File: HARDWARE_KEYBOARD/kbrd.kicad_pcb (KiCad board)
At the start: 2 copper layers, 70 x 50 mm, 24 parts, among them J1 USB_C_Receptacle_USB2.0_16P, J2 SWD, SW1 SW_SPST, SW2 SW_SPST, SW3 SW_SPST, SW4 SW_SPST, U1 STM32F103C8Tx, U2 AP2210N-3.3TRG1, Y1 Crystal_GND24

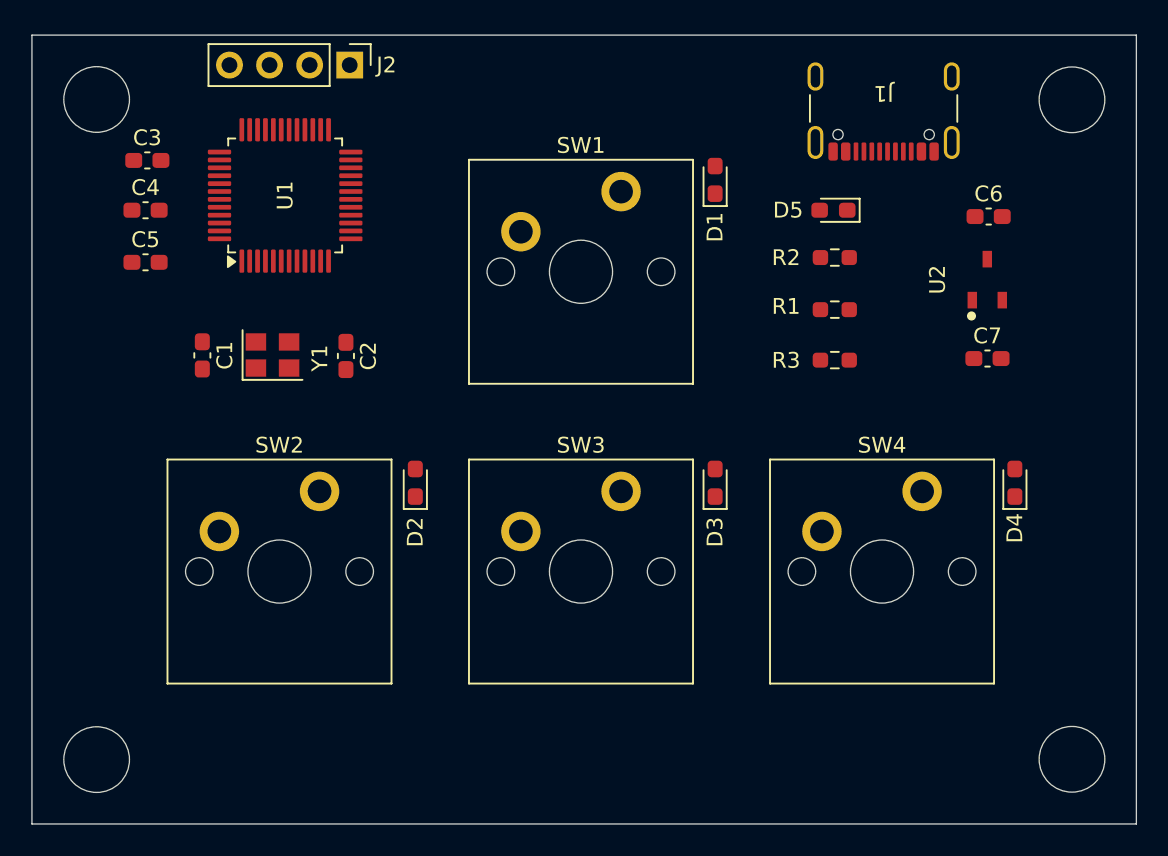
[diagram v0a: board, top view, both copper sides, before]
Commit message: Updated PCB & schematic
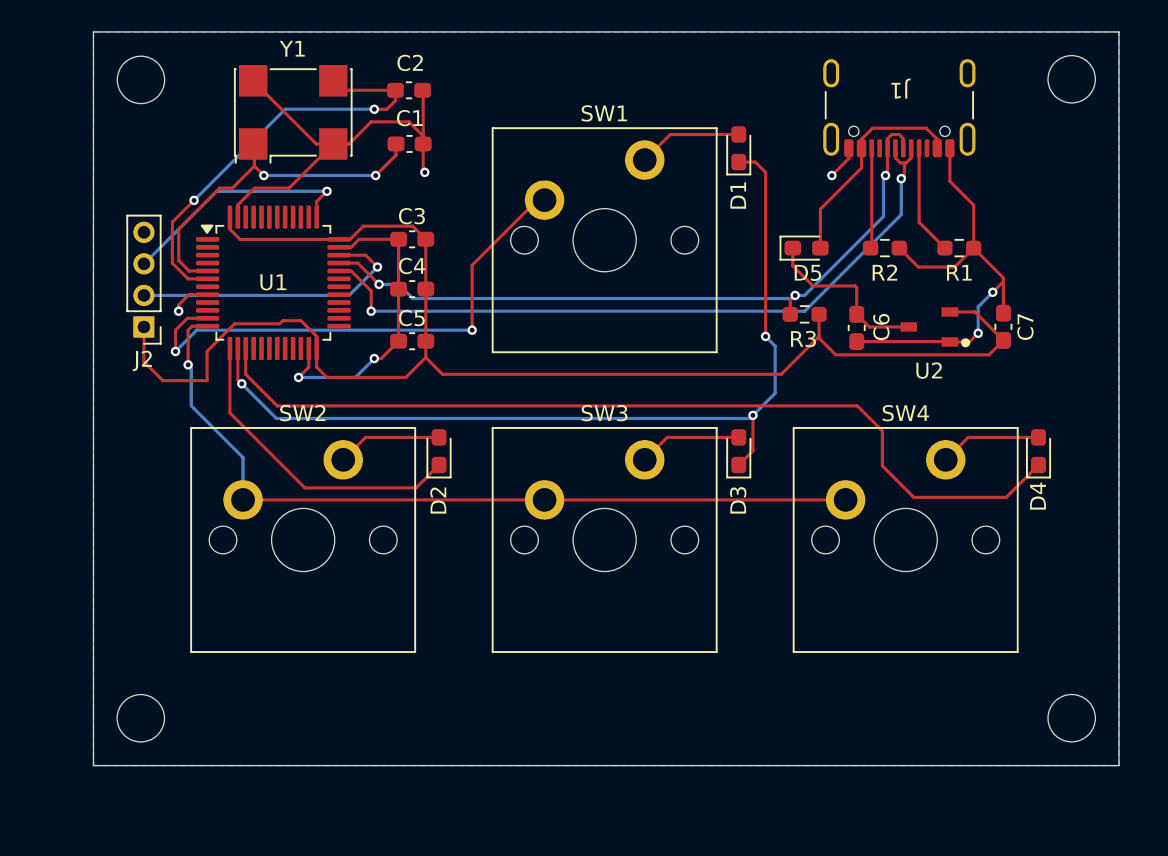
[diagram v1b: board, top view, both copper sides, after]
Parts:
- J2: footprint Connector_PinHeader_2.54mm:PinHeader_1x04_P2.54mm_Vertical -> Connector_PinHeader_2.00mm:PinHeader_1x04_P2.00mm_Vertical
- Y1: footprint Oscillator:Oscillator_SMD_Abracon_ASE-4Pin_3.2x2.5mm -> Oscillator:Oscillator_SMD_Abracon_ASV-4Pin_7.0x5.1mm
- moved J2 21.1 mm to (125.6, 90.8), turned to 180 degrees
- moved C1 18.8 mm to (142.4, 79.2), turned to 0 degrees
- moved C4 17.6 mm to (142.6, 88.4)
- moved C5 17.6 mm to (142.6, 91.7)
- moved C3 17.5 mm to (142.6, 85.2)
- moved C2 17.3 mm to (142.4, 75.8), turned to 0 degrees
- moved Y1 15.4 mm to (135.1, 77.2)
- moved C6 10.9 mm to (170.8, 90.9), turned to 90 degrees
- moved R1 8.80 mm to (177.3, 85.8), turned to 180 degrees
- moved U1 5.59 mm to (133.8, 88.0), turned to 0 degrees
- moved U2 4.74 mm to (175.4, 90.8), turned to 180 degrees
- moved R3 3.47 mm to (167.5, 90.0)
- moved R2 3.23 mm to (172.6, 85.8), turned to 180 degrees
- moved D5 2.94 mm to (167.6, 85.8), turned to 0 degrees
- moved D1 2.50 mm to (163.3, 79.5)
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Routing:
- net +3.3V: track 0.00 -> 92.7 mm
- net GND: track 0.00 -> 81.8 mm, vias 0 -> 7
- net /COL2: track 0.00 -> 57.5 mm, vias 0 -> 3
- net /COL3: track 0.00 -> 57.3 mm
- net /ROW2: track 0.00 -> 51.7 mm, vias 0 -> 1
- net /PA11: track 0.00 -> 46.0 mm, vias 0 -> 2
- net /PA12: track 0.00 -> 45.8 mm, vias 0 -> 3
- net /ROW1: track 0.00 -> 33.5 mm, vias 0 -> 2
- net /OSC_OUT: track 0.00 -> 27.4 mm, vias 0 -> 2
- net /OSC_IN: track 0.00 -> 21.5 mm, vias 0 -> 2
- net /COL1: track 0.00 -> 19.9 mm
- net /SWDIO: track 0.00 -> 18.3 mm, vias 0 -> 1
- net /SWCLK: track 0.00 -> 15.4 mm, vias 0 -> 1
- net Net-(D5-A): track 0.00 -> 13.9 mm
- net VCC: track 0.00 -> 11.1 mm
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- added copper zone on B.Cu, net GND
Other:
- board size 70 x 50 mm -> 65 x 46.5 mm
